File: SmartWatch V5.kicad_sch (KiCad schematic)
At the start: 61 parts, among them J1 10118192-0001LF, J10 TestPad, J8 TestPad, J9 TestPad, Q1 FDN340P, Q2 MMBT3904, Q3 MMBT3904, Q5 FDN028N20, Q6 FDN028N20, SW1 EVQ-P7J01P, SW2 EVQ-P7J01P, U1 MAX17260, U10 TSC2003IPWR, U2 FT231XQ, U3 LP5912-3.3DRVT, U4 ADXL335BCPZ-RL, U5 MCP73832-2-OT, U6 ESP32-WROOM-32

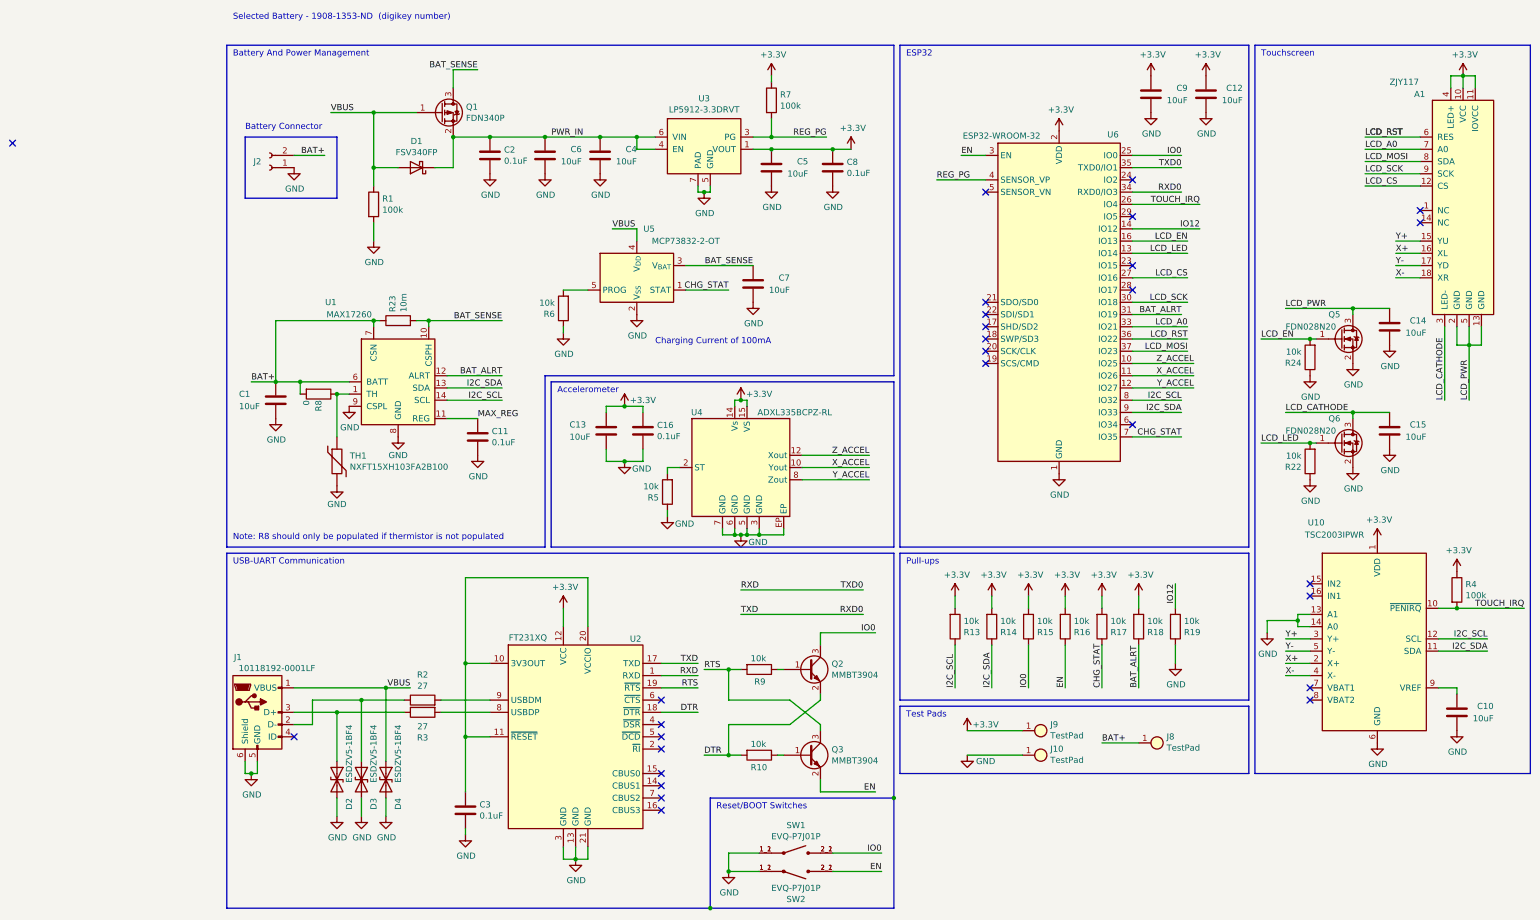
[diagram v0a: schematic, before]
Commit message: revert kicad_sch for testing
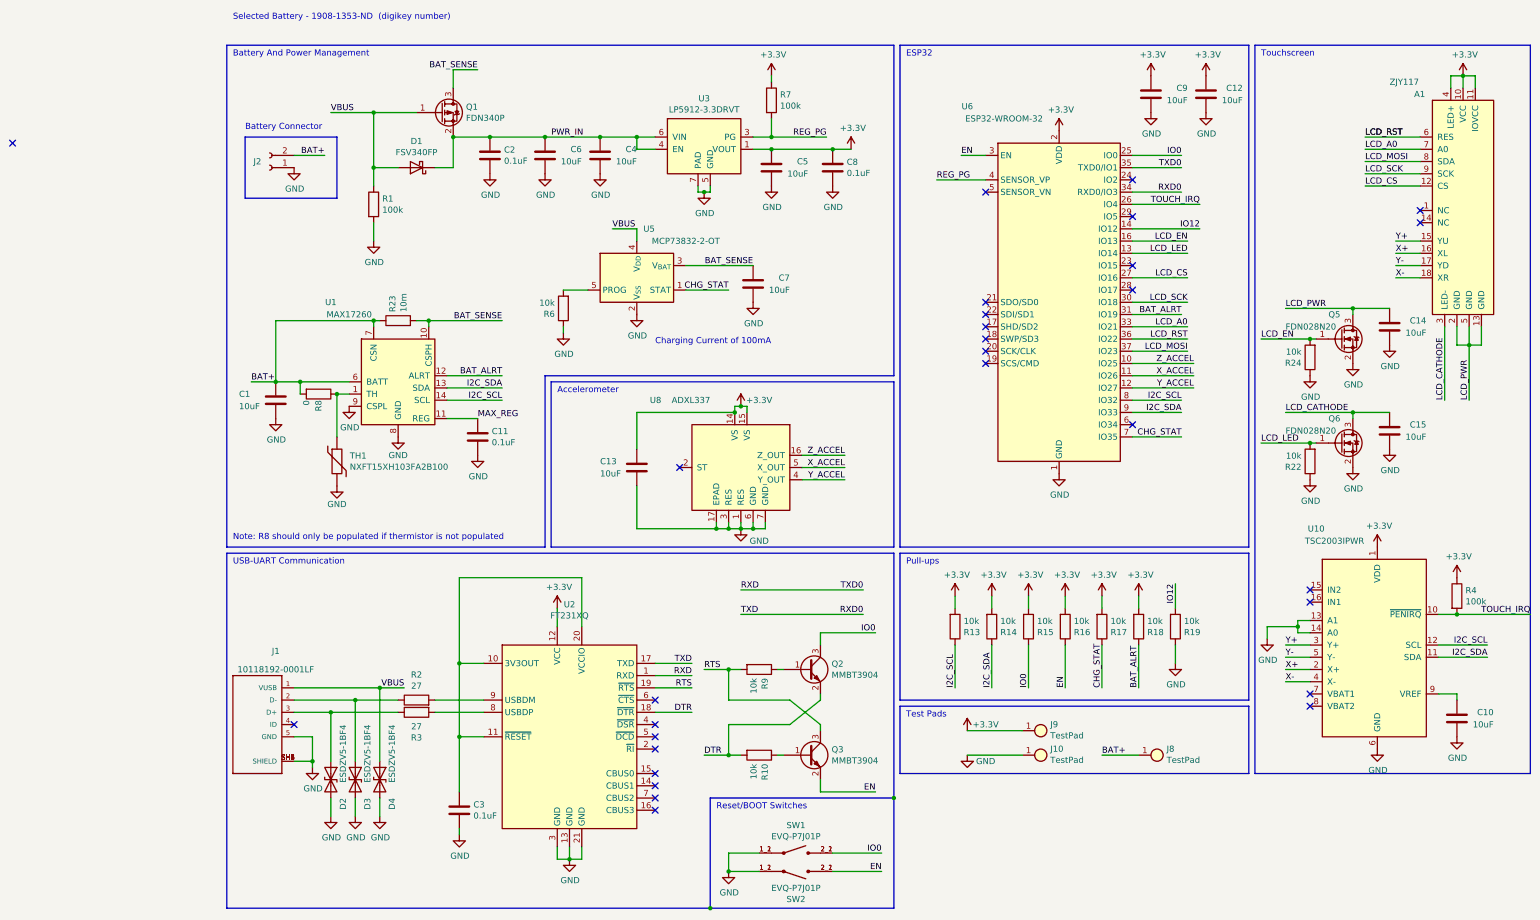
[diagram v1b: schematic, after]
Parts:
- removed C16: 0.1uF, Capacitor_SMD:C_0603_1608Metric, symbol Device:C
- removed R5: 10k, Resistor_SMD:R_0603_1608Metric, symbol Device:R
- removed U4: ADXL335BCPZ-RL, Package_CSP:Analog_LFCSP-16-1EP_4x4mm_P0.65mm_EP2.35x2.35mm, symbol symbol_library:ADXL335BCPZ-RL
- added U8: ADXL337, CustomFootprints:ADXL337BCPZ-RL, symbol CustomParts:ADXL337
- J1: symbol Connector:USB_B_Micro -> CustomParts:10118192-0001LF
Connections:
- net +3.3V: now also U8.14 (VS), U8.15 (VS)
- net GND: now also J1.SH1 (SHIELD), J1.SH2 (SHIELD), J1.SH3 (SHIELD), J1.SH4 (SHIELD), J1.SH5 (SHIELD), J1.SH6 (SHIELD), U8.1 (RES), U8.17 (EPAD), U8.3 (RES), U8.6 (GND), U8.7 (GND); no longer J1.6 (Shield)
- net X_ACCEL: now also U8.5 (X_OUT)
- net Y_ACCEL: now also U8.4 (Y_OUT)
- net Z_ACCEL: now also U8.16 (Z_OUT)
- no-connect marks 28 -> 29
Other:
- moved on the sheet: C10, C13, C3, D2, D3, D4, J8, R2, R3, R4, U10, U2
